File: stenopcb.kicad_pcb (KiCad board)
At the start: 2 copper layers, 100.3 x 95.2 mm, 83 parts, among them K1 MAIN_RIGHT_TO_VOWELS_RIGHT, K2 MAIN_LEFT_TO_VOWELS_LEFT, K3 VOWELS_RIGHT_IN, K4 VOWELS_LEFT_IN, P1 MAIN_RIGHT_IN, P2 MAIN_RIGHT_TO_MAIN_LEFT, P3 MAIN_LEFT_IN, SW1 SPST, SW10 SPST, SW11 SPST, SW12 SPST, SW13 SPST, SW14 SPST, SW15 SPST, SW16 SPST, SW17 SPST, SW18 SPST, SW19 SPST, SW2 SPST, SW20 SPST, SW21 SPST, SW22 SPST, SW23 SPST, SW24 SPST, SW25 SPST, SW26 SPST, SW27 SPST, SW28 SPST, SW29 SPST, SW3 SPST, SW30 SPST, SW4 SPST, SW5 SPST, SW6 SPST, SW7 SPST, SW8 SPST, SW9 SPST

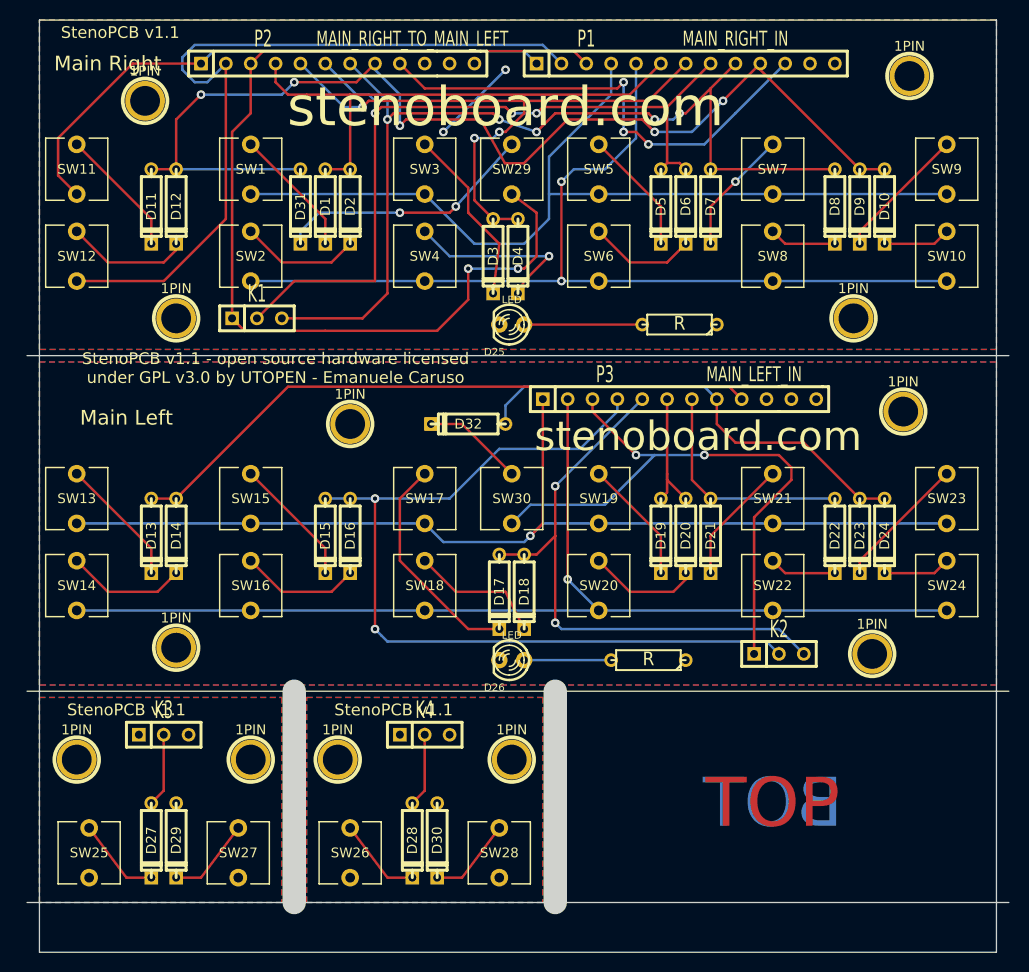
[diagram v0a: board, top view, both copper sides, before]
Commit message: my changes.. don't remember for what anymore :/
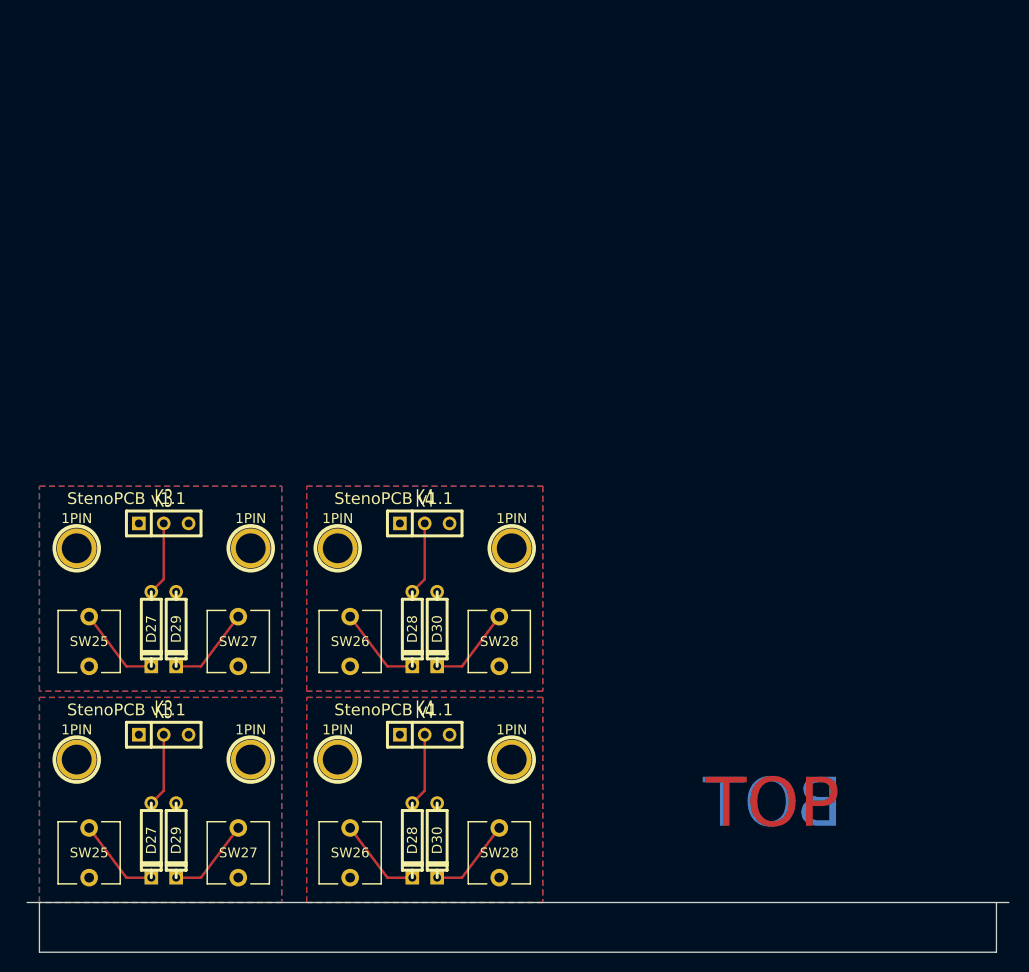
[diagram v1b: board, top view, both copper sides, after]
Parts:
- removed the 1PIN at (121.9, 70.5)
- removed the 1PIN at (125.1, 92.7)
- removed the 1PIN at (200.0, 67.9)
- removed the 1PIN at (194.3, 92.7)
- removed the 1PIN at (142.9, 103.5)
- removed the 1PIN at (125.1, 126.4)
- removed the 1PIN at (199.4, 102.2)
- removed the 1PIN at (196.2, 127.0)
- removed D1, D10, D11, D12, D13, D14, D15, D16, D17, D18, D19, D2, D20, D21, D22, D23, D24, D3, D31, D32, D4, D5, D6, D7, D8, D9: DIODE, D3
- removed D25, D26: LED, LED-3MM
- removed K1: MAIN_RIGHT_TO_VOWELS_RIGHT, SIL-3
- removed K2: MAIN_LEFT_TO_VOWELS_LEFT, SIL-3
- removed P1: MAIN_RIGHT_IN, SIL-13
- removed P2: MAIN_RIGHT_TO_MAIN_LEFT, SIL-12
- removed P3: MAIN_LEFT_IN, SIL-12
- removed R1, R2: R, R3
- removed SW1, SW10, SW11, SW12, SW13, SW14, SW15, SW16, SW17, SW18, SW19, SW2, SW20, SW21, SW22, SW23, SW24, SW29, SW3, SW30, SW4, SW5, SW6, SW7, SW8, SW9: SPST, EVQ-P0E07K
- added 1PIN: P***, 1pin, F.Cu at (159.4, 116.2)
- added 1PIN: P***, 1pin, F.Cu at (141.6, 116.2)
- added 1PIN: P***, 1pin, F.Cu at (132.7, 116.2)
- added 1PIN: P***, 1pin, F.Cu at (114.9, 116.2)
- added D27: DIODE, D3, F.Cu at (122.6, 124.5)
- added D28: DIODE, D3, F.Cu at (149.2, 124.5)
- added D29: DIODE, D3, F.Cu at (125.1, 124.5)
- added D30: DIODE, D3, F.Cu at (151.8, 124.5)
- added K3: VOWELS_RIGHT_IN, SIL-3, F.Cu at (123.8, 113.7)
- added K4: VOWELS_LEFT_IN, SIL-3, F.Cu at (150.5, 113.7)
- added SW25: SPST, EVQ-P0E07K, F.Cu at (116.2, 125.7)
- added SW26: SPST, EVQ-P0E07K, F.Cu at (142.9, 125.7)
- added SW27: SPST, EVQ-P0E07K, F.Cu at (131.4, 125.7)
- added SW28: SPST, EVQ-P0E07K, F.Cu at (158.1, 125.7)
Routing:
- net /COL_4: track 113.0 -> 0.00 mm, vias 5 -> 0
- net /L_ROW_1: track 111.8 -> 0.00 mm, vias 1 -> 0
- net /ROW_2: track 106.4 -> 0.00 mm, vias 2 -> 0
- net /L_ROW_0: track 105.0 -> 0.00 mm, vias 1 -> 0
- net /ROW_4: track 98.4 -> 0.00 mm, vias 2 -> 0
- net /COL_3: track 97.6 -> 0.00 mm, vias 5 -> 0
- net /ROW_3: track 92.8 -> 0.00 mm
- net /L_COL_0: track 91.1 -> 0.00 mm, vias 2 -> 0
- net /COL_2: track 84.4 -> 0.00 mm, vias 3 -> 0
- net /ROW_1: track 80.8 -> 0.00 mm
- net /L_COL_5: track 65.6 -> 0.00 mm
- net /L_ROW_2: track 62.1 -> 0.00 mm, vias 2 -> 0
- net /COL_1: track 62.0 -> 0.00 mm, vias 3 -> 0
- net /L_COL_1: track 59.8 -> 0.00 mm, vias 2 -> 0
- net /ROW_0: track 59.6 -> 0.00 mm
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- removed copper zone on B.Cu, net /GND
- removed copper zone on F.Cu, net /LED
- removed copper zone on B.Cu, net /L_GND
- removed copper zone on F.Cu, net /L_LED
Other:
- board size 100.3 x 95.2 mm -> 100.3 x 5.1 mm
- board text removed: "Main Left"
- board text removed: "Main Right"
- board text removed: "StenoPCB v1.1 - open source hardware licensed under GPL v3.0 by UTOPEN - Emanuele Caruso"
- board text removed: "stenoboard.com"
